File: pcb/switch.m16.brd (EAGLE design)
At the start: 78.9 x 77.8 mm, 34 parts

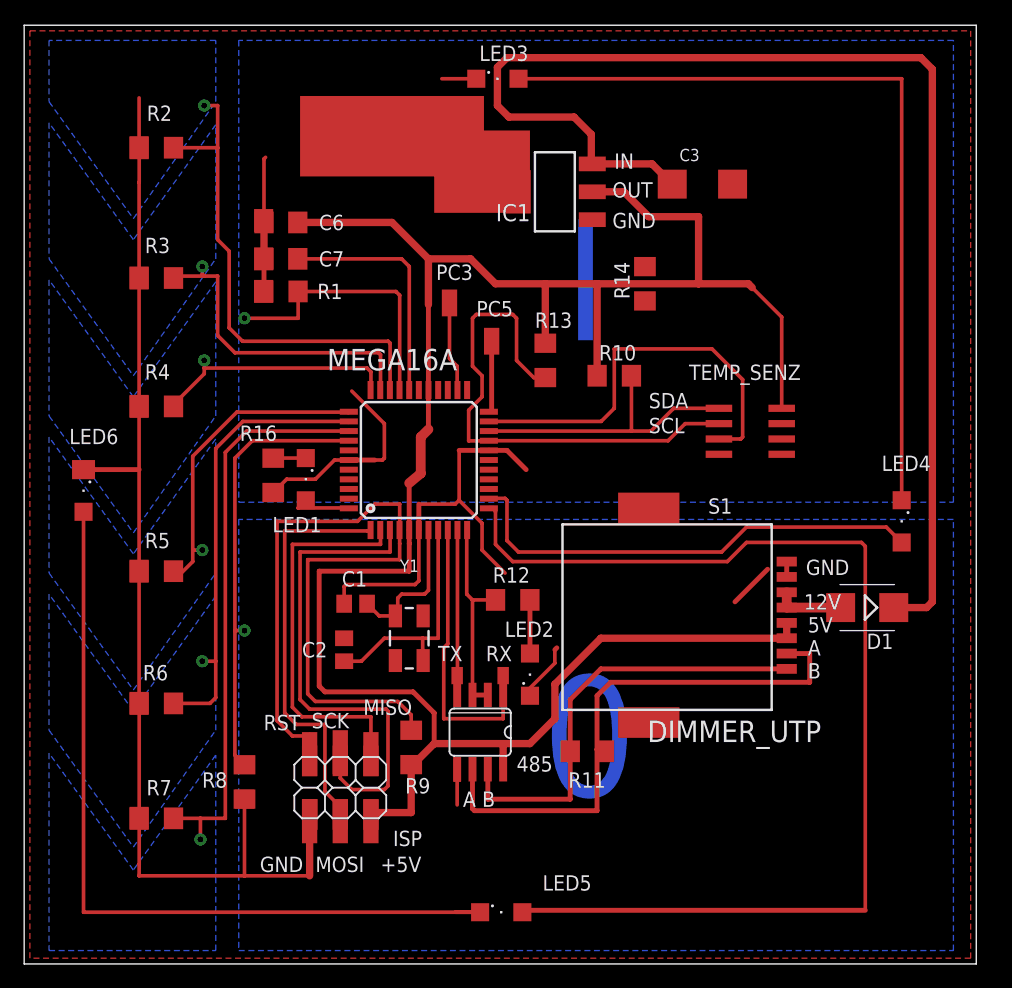
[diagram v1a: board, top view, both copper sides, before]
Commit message: initial add light
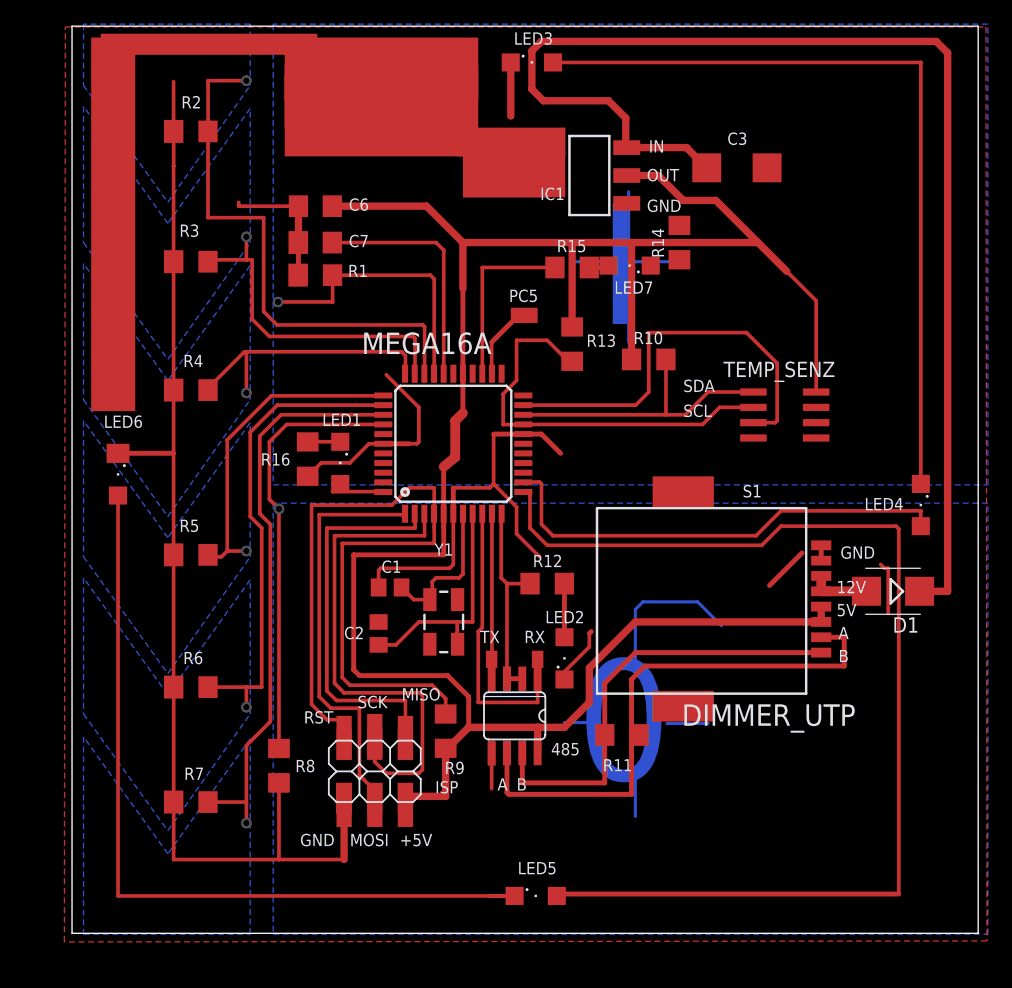
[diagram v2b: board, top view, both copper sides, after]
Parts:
- added LED7: (no value), led:SML1206
- added R15: 4k7, rcl:R1206
- R14: value 10k -> 0
- moved R14 4.45 mm to (50.3, 57.2)
- moved LED3 3.16 mm to (38.1, 72.2)
- moved 485 3.16 mm to (36.7, 18.0)
- moved C3 3.16 mm to (55.1, 63.4)
- moved LED1 3.16 mm to (22.2, 39.0)
- moved LED2 3.16 mm to (40.8, 22.8)
- moved R16 3.16 mm to (19.5, 39.3)
- moved R9 3.16 mm to (31.0, 16.7)
- moved TEMP_SENZ 3.16 mm to (59.1, 42.9)
- moved LED6 3.16 mm to (3.81, 38.0)
- moved ISP 3.16 mm to (22.5, 14.7)
- moved R11 3.16 mm to (45.6, 16.4)
- moved R3 3.16 mm to (9.84, 55.6)
- moved R4 3.16 mm to (9.84, 45.0)
- moved R8 3.16 mm to (17.1, 13.9)
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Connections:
- new net N$13: LED7.A, R15.2
- new net N$9: MEGA16A.25, R15.1
- new net PC5: MEGA16A.24
- net GND: now also LED7.C
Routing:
- net N$6: track 36.9 -> 59.6 mm
- net N$5: track 23.6 -> 44.7 mm
- net N$9: track 0.00 -> 14.8 mm
- net GND: track 175.8 -> 187.4 mm
- net N$26: track 7.88 -> 0.00 mm
- net N$10: track 43.1 -> 35.5 mm
- net N$44: track 1.11 -> 7.54 mm
- net N$14: track 5.72 -> 0.00 mm
- net PC5: track 0.00 -> 5.33 mm
- net N$4: track 40.2 -> 37.3 mm
- net N$31: track 20.4 -> 22.9 mm
- net N$8: track 37.4 -> 39.6 mm
- net N$3: track 106.0 -> 103.8 mm
- net VCC: track 183.3 -> 185.4 mm
- net N$13: track 0.00 -> 1.75 mm
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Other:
- board size 78.9 x 77.8 mm -> 75.1 x 75.2 mm
- board text removed: "PC3"
